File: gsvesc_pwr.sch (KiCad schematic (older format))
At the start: 36 parts, among them J10 PHASE_C, J11 PHASE_A, J12 NTC, J13 PHASE_B, Q1 NVMFS5C604, Q2 NVMFS5C604, Q3 NVMFS5C604, Q4 NVMFS5C604, Q5 NVMFS5C604, Q6 NVMFS5C604, U4 AD8418, U5 AD8418, U6 AD8418

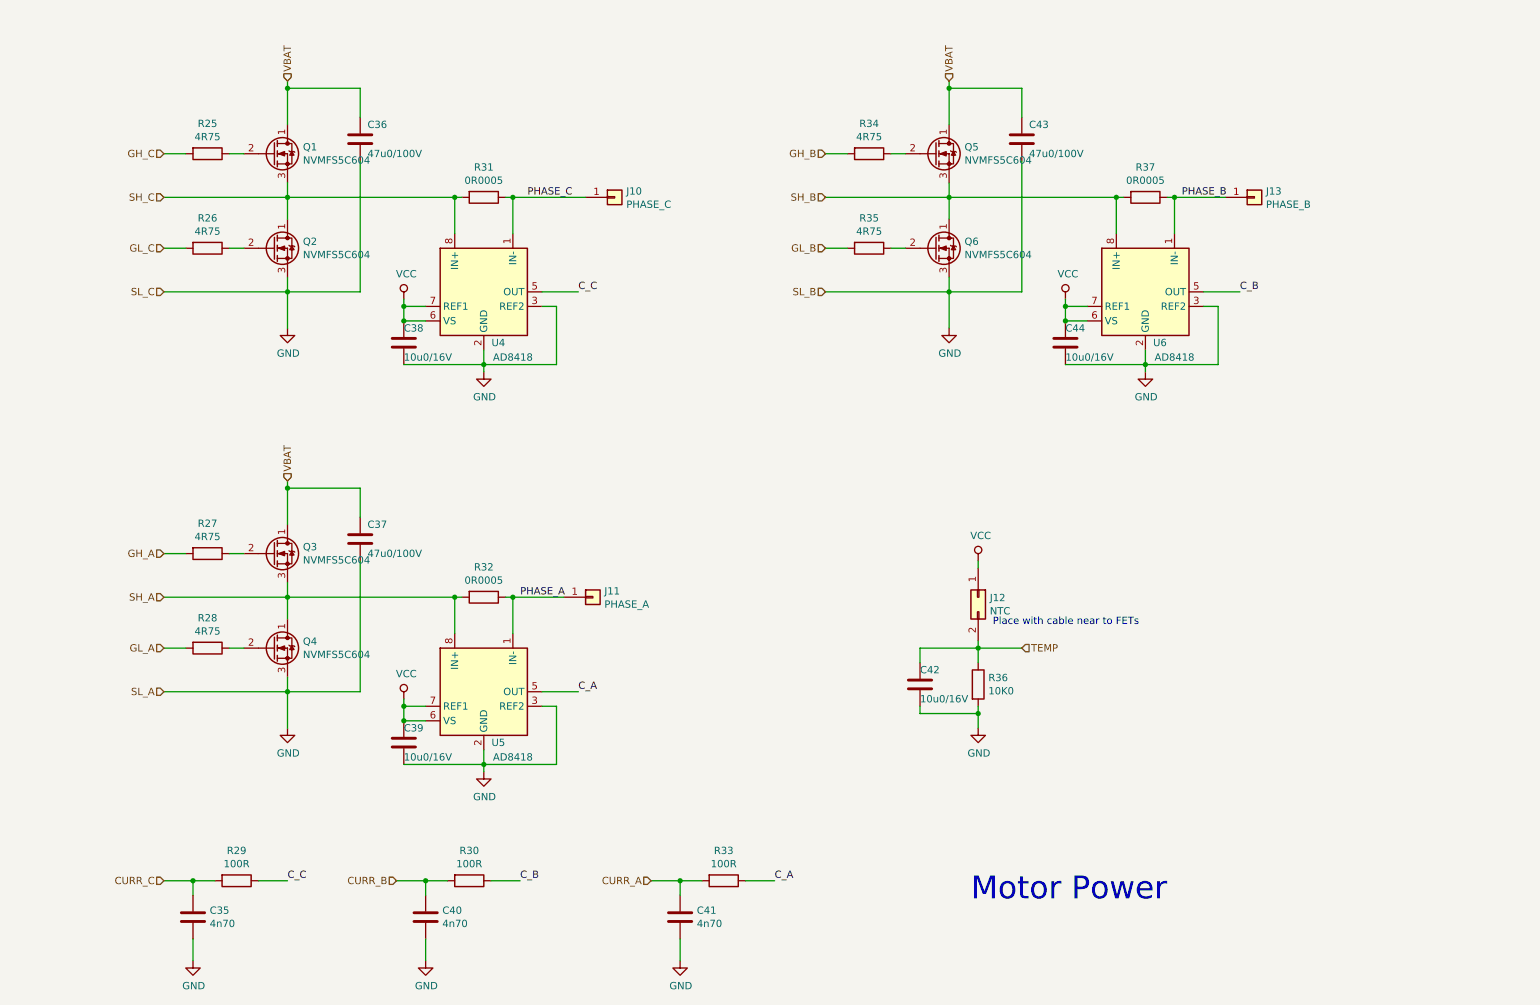
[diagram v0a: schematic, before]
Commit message: test
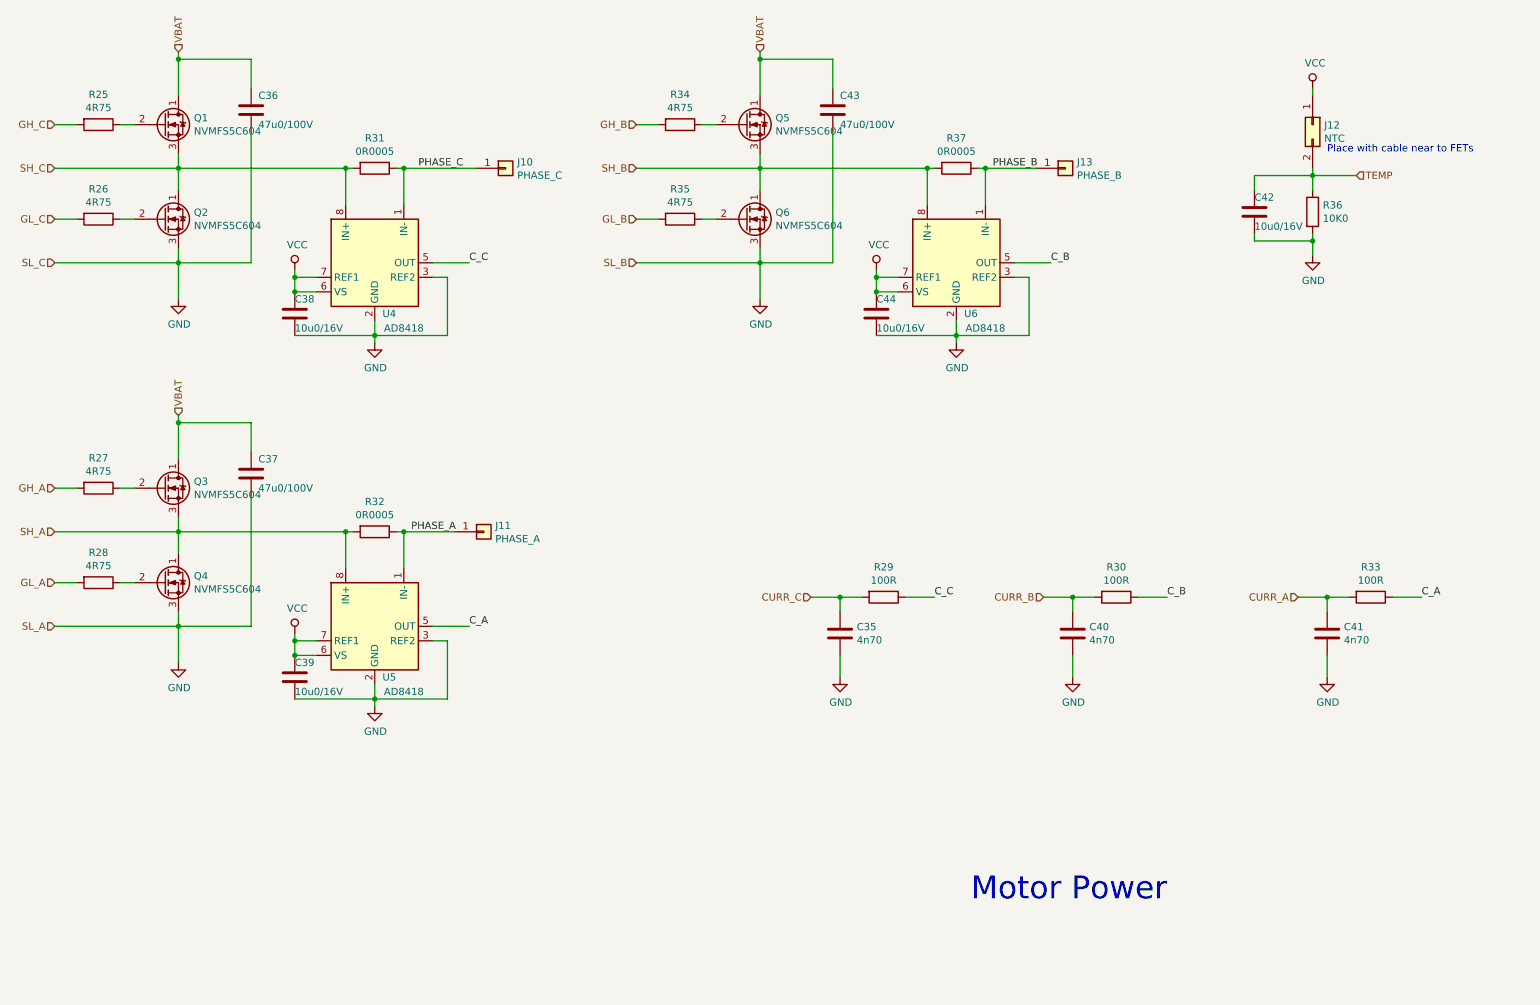
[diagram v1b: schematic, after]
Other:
- moved on the sheet: C35, C36, C37, C38, C39, C40, C41, C42, C43, C44, J10, J11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
